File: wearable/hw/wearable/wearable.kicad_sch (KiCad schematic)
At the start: 103 parts, among them IC1 LM4041CILPR, J2 Conn_02x05_Odd_Even, J3 Interrupts, J4 Data, J5 Data, J8 USBC Charger, SW1 SW_Toggle, U1 LT3042xMSE, U2 BNO080, U3 nRF54L15-QFXX, U4 MAX77659AENV+, U5 ADS1299IPAG, Y1 32MHz, Y2 32.768kHz, Y3 32.768kHz

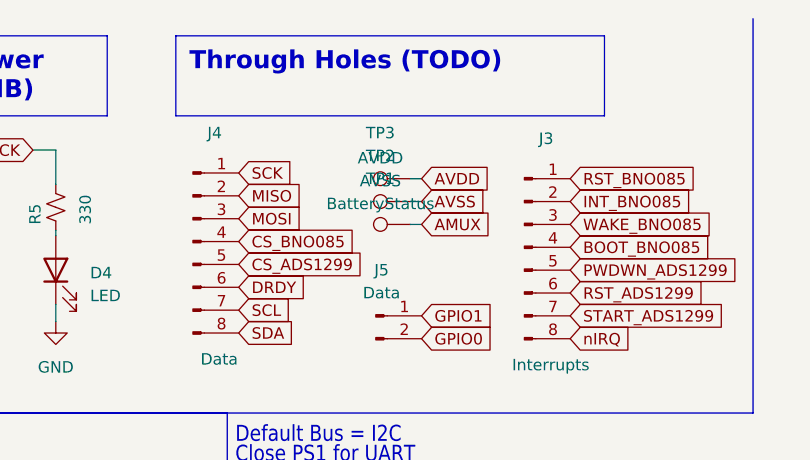
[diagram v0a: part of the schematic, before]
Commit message: More layout progress and some fun stuff
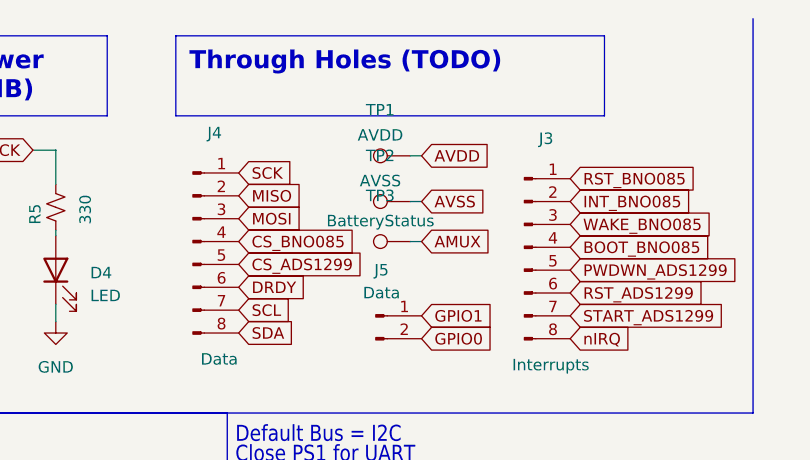
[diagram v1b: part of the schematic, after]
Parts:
- renumbered TP3 to TP1, TP1 to TP3
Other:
- moved on the sheet: TP1, TP3
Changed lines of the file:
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@@
 	(wire
 		(pts
-			(xy 222.25 22.86) (xy 223.52 22.86)
+			(xy 222.25 24.765) (xy 223.52 24.765)
 		)
 		(stroke
@@
 	(wire
 		(pts
-			(xy 222.25 17.78) (xy 223.52 17.78)
+			(xy 222.25 15.24) (xy 223.52 15.24)
 		)
 		(stroke
@@
 	(global_label "AMUX"
 		(shape input)
-		(at 223.52 22.86 0)
+		(at 223.52 24.765 0)
 		(fields_autoplaced yes)
 		(effects
@@
 		)
 		(property "Intersheetrefs" "${INTERSHEET_REFS}"
-			(at 231.5852 22.86 0)
+			(at 231.5852 24.765 0)
 			(effects
 				(font
@@
 	(global_label "AVDD"
 		(shape input)
-		(at 223.52 17.78 0)
+		(at 223.52 15.24 0)
 		(fields_autoplaced yes)
 		(effects
@@
 		)
 		(property "Intersheetrefs" "${INTERSHEET_REFS}"
-			(at 231.2224 17.78 0)
+			(at 231.2224 15.24 0)
 			(effects
 				(font
@@
 	(symbol
 		(lib_id "Connector:TestPoint")
-		(at 222.25 17.78 90)
+		(at 222.25 15.24 90)
 		(unit 1)
 		(exclude_from_sim no)
@@
 		(on_board yes)
 		(dnp no)
-		(property "Reference" "TP3"
-			(at 218.948 12.7 90)
+		(property "Reference" "TP1"
+			(at 218.948 10.16 90)
 			(effects
 				(font
@@
 		)
 		(property "Value" "AVDD"
-			(at 218.948 15.494 90)
+			(at 218.948 12.954 90)
 			(effects
 				(font
@@
 		)
 		(property "Footprint" "TestPoint:TestPoint_Bridge_Pitch2.0mm_Drill0.7mm"
-			(at 222.25 12.7 0)
+			(at 222.25 10.16 0)
 			(effects
 				(font
@@
 		)
 		(property "Datasheet" "~"
-			(at 222.25 12.7 0)
+			(at 222.25 10.16 0)
 			(effects
 				(font
@@
 		)
 		(property "Description" "test point"
-			(at 222.25 17.78 0)
+			(at 222.25 15.24 0)
 			(effects
 				(font
@@
 			(project "wearable"
 				(path "/eeafcd59-7fa6-43d8-bb03-b6b192c7124f"
-					(reference "TP3")
+					(reference "TP1")
 					(unit 1)
 				)
@@
 	(symbol
 		(lib_id "Connector:TestPoint")
-		(at 222.25 22.86 90)
+		(at 222.25 24.765 90)
 		(unit 1)
 		(exclude_from_sim no)
@@
 		(on_board yes)
 		(dnp no)
-		(property "Reference" "TP1"
-			(at 218.948 17.78 90)
+		(property "Reference" "TP3"
+			(at 218.948 19.685 90)
 			(effects
 				(font
@@
 		)
 		(property "Value" "BatteryStatus"
-			(at 218.948 20.574 90)
+			(at 218.948 22.479 90)
 			(effects
 				(font
@@
 		)
 		(property "Footprint" "TestPoint:TestPoint_Bridge_Pitch2.0mm_Drill0.7mm"
-			(at 222.25 17.78 0)
+			(at 222.25 19.685 0)
 			(effects
 				(font
@@
 		)
 		(property "Datasheet" "~"
-			(at 222.25 17.78 0)
+			(at 222.25 19.685 0)
 			(effects
 				(font
@@
 		)
 		(property "Description" "test point"
-			(at 222.25 22.86 0)
+			(at 222.25 24.765 0)
 			(effects
 				(font
@@
 			(project ""
 				(path "/eeafcd59-7fa6-43d8-bb03-b6b192c7124f"
-					(reference "TP1")
+					(reference "TP3")
 					(unit 1)
 				)
